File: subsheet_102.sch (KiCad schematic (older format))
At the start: 54 parts, among them J6 DIN13S, Q10 2N3904, Q2 2N3904, Q3 Q_NPN_CBE, Q4 2N3904, Q5 2N3904, U31 ST_SHIFTER_PHY

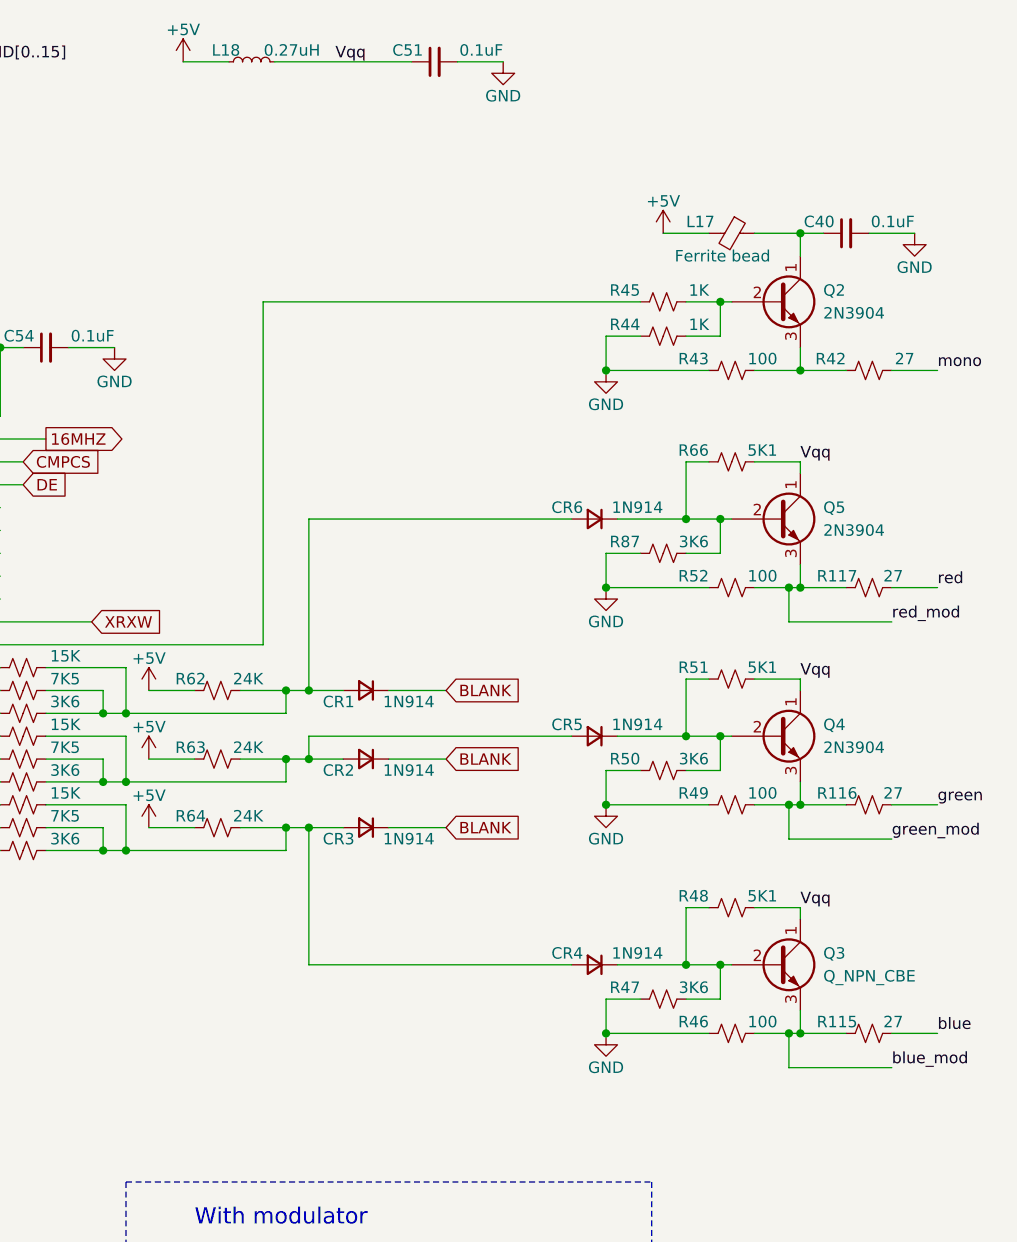
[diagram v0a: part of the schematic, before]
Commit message: Wired 'Vqq' together to remove label, add missing annotations, assigned footprints
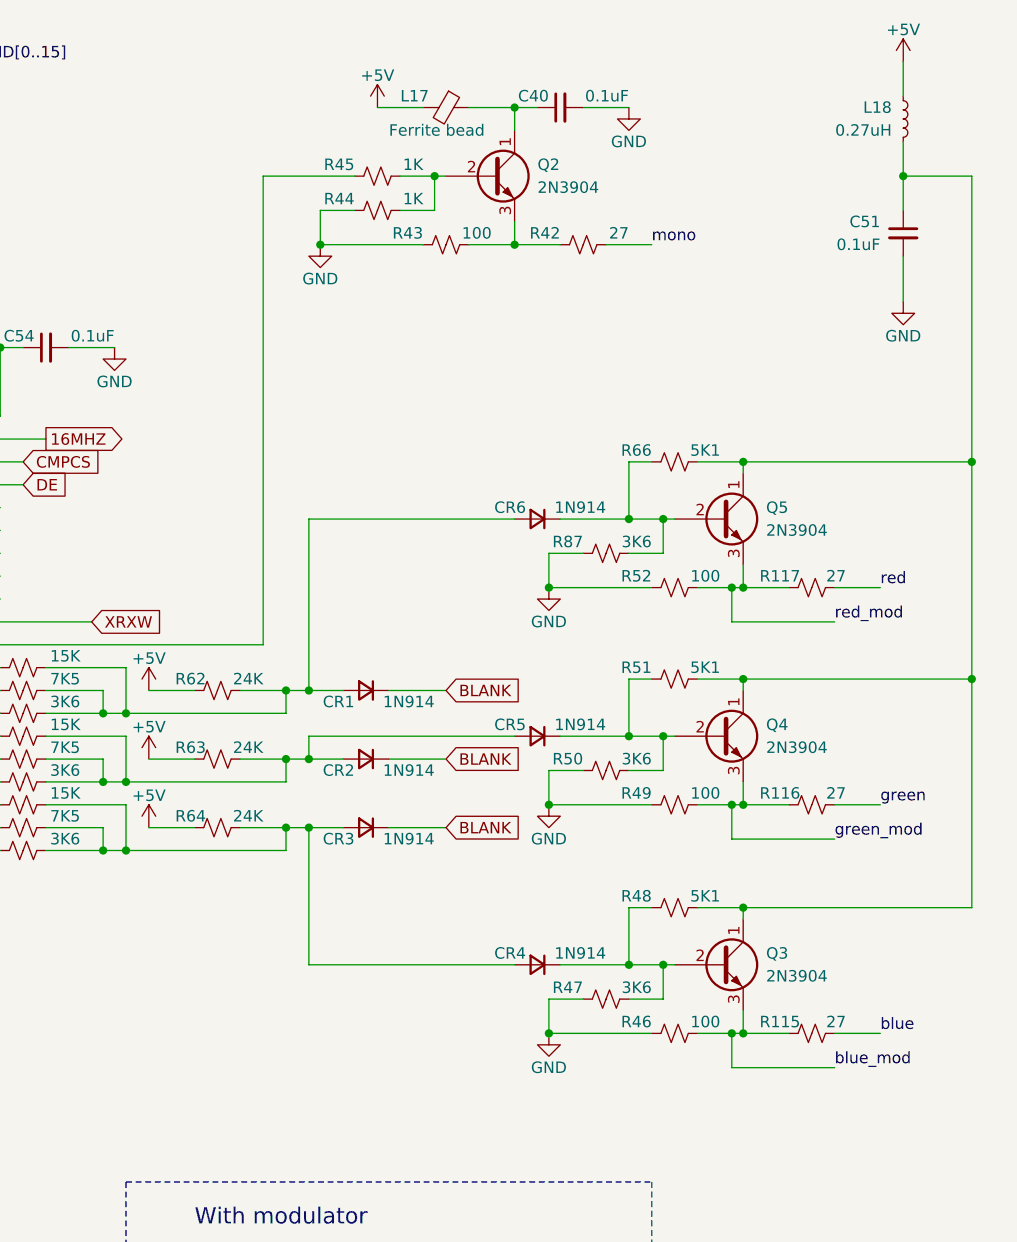
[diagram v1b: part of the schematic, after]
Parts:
- CR1, CR10, CR2, CR3, CR4, CR5, CR6, CR9: footprint (none) -> commons-passives_THT:Passive_THT_diode_W2.54mm_L15.24mm
- J6: footprint (none) -> atari-interconnect:socket-din-13
- JMOD1: footprint (none) -> Connector_PinSocket_2.54mm:PinSocket_1x10_P2.54mm_Vertical
- Q10, Q2, Q4, Q5: footprint (none) -> Package_TO_SOT_THT:TO-92L_Inline_Wide
- Q3: value Q_NPN_CBE -> 2N3904; footprint (none) -> Package_TO_SOT_THT:TO-92L_Inline_Wide
- R115, R116, R117, R127, R129, R130, R131, R42, R43, R44, R45, R46, R47, R48, R49, R50, R51, R52, R53, R54, R55, R56, R57, R58, R59, R60, R61, R62, R63, R64, R66, R87: footprint (none) -> commons-passives_THT:Passive_THT_resistor_W2.54mm_L15.24mm
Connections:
- net Vqq: no longer names the net of C51.1, L18.2, Q3.1 (C), Q4.1 (C), Q5.1 (C), R48.2, R51.2, R66.2
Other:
- moved on the sheet: C40, C51, CR4, CR5, CR6, L17, L18, Q2, Q3, Q4, Q5, R115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
